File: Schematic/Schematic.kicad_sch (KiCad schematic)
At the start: 17 parts, among them J1 XT60-M, T1 Telemetry, U1 Matek PDB, U2 DRV8838

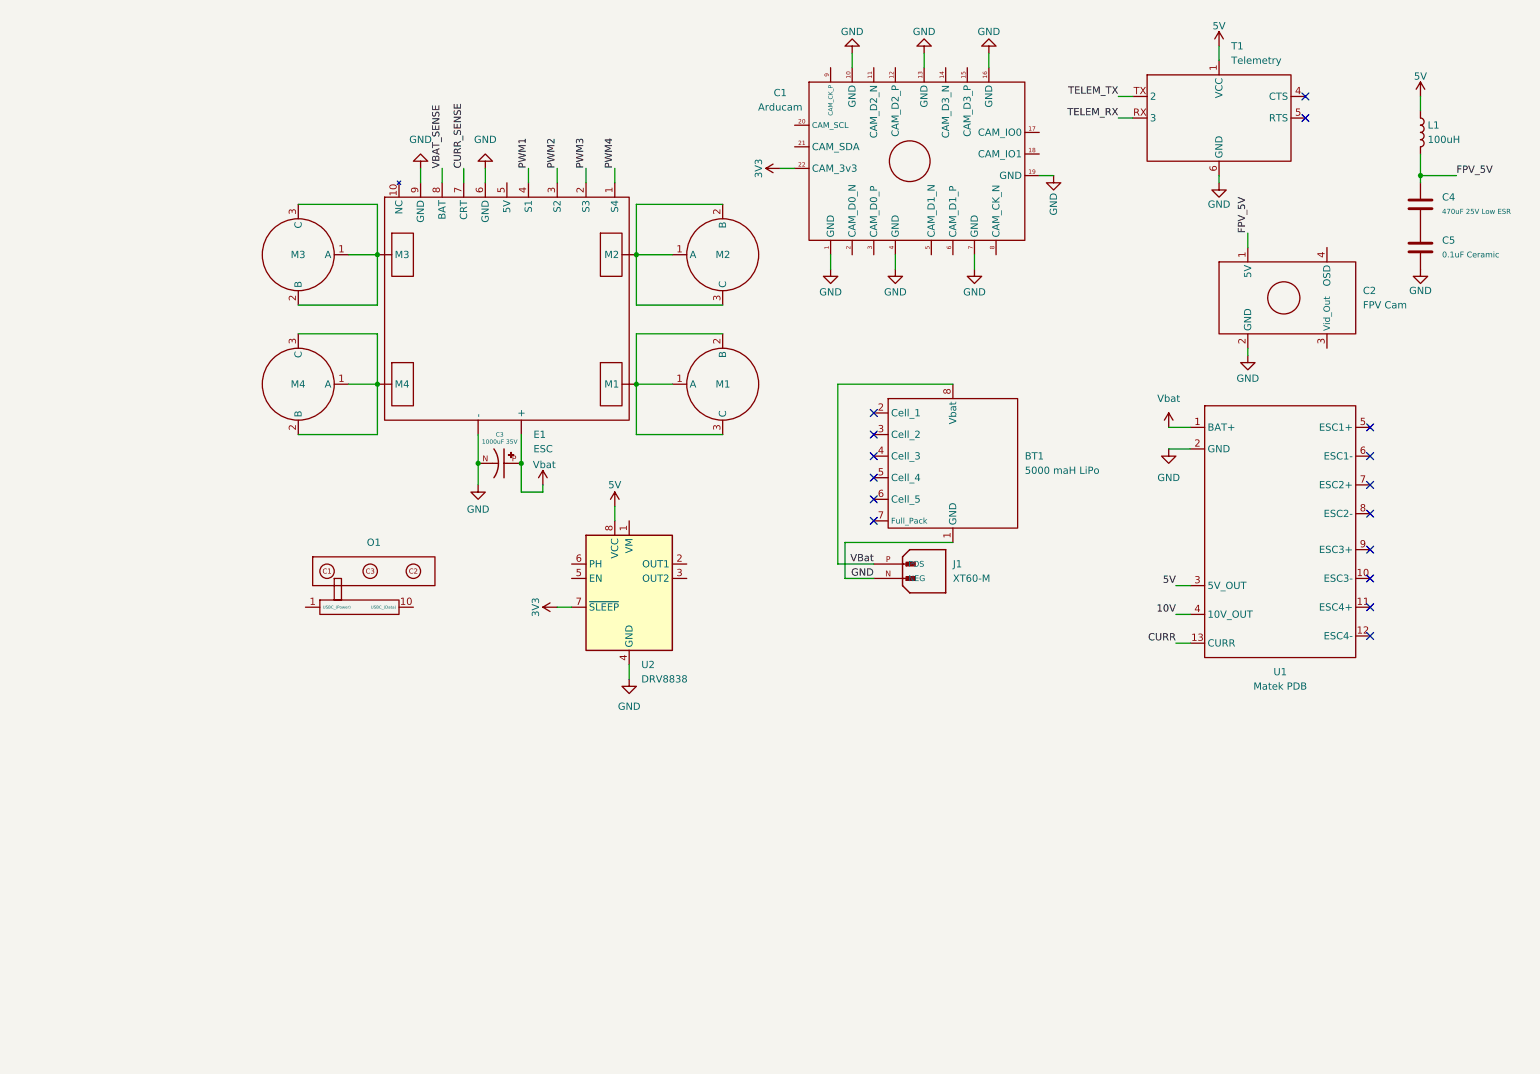
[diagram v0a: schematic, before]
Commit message: 6x and Jetson schematic
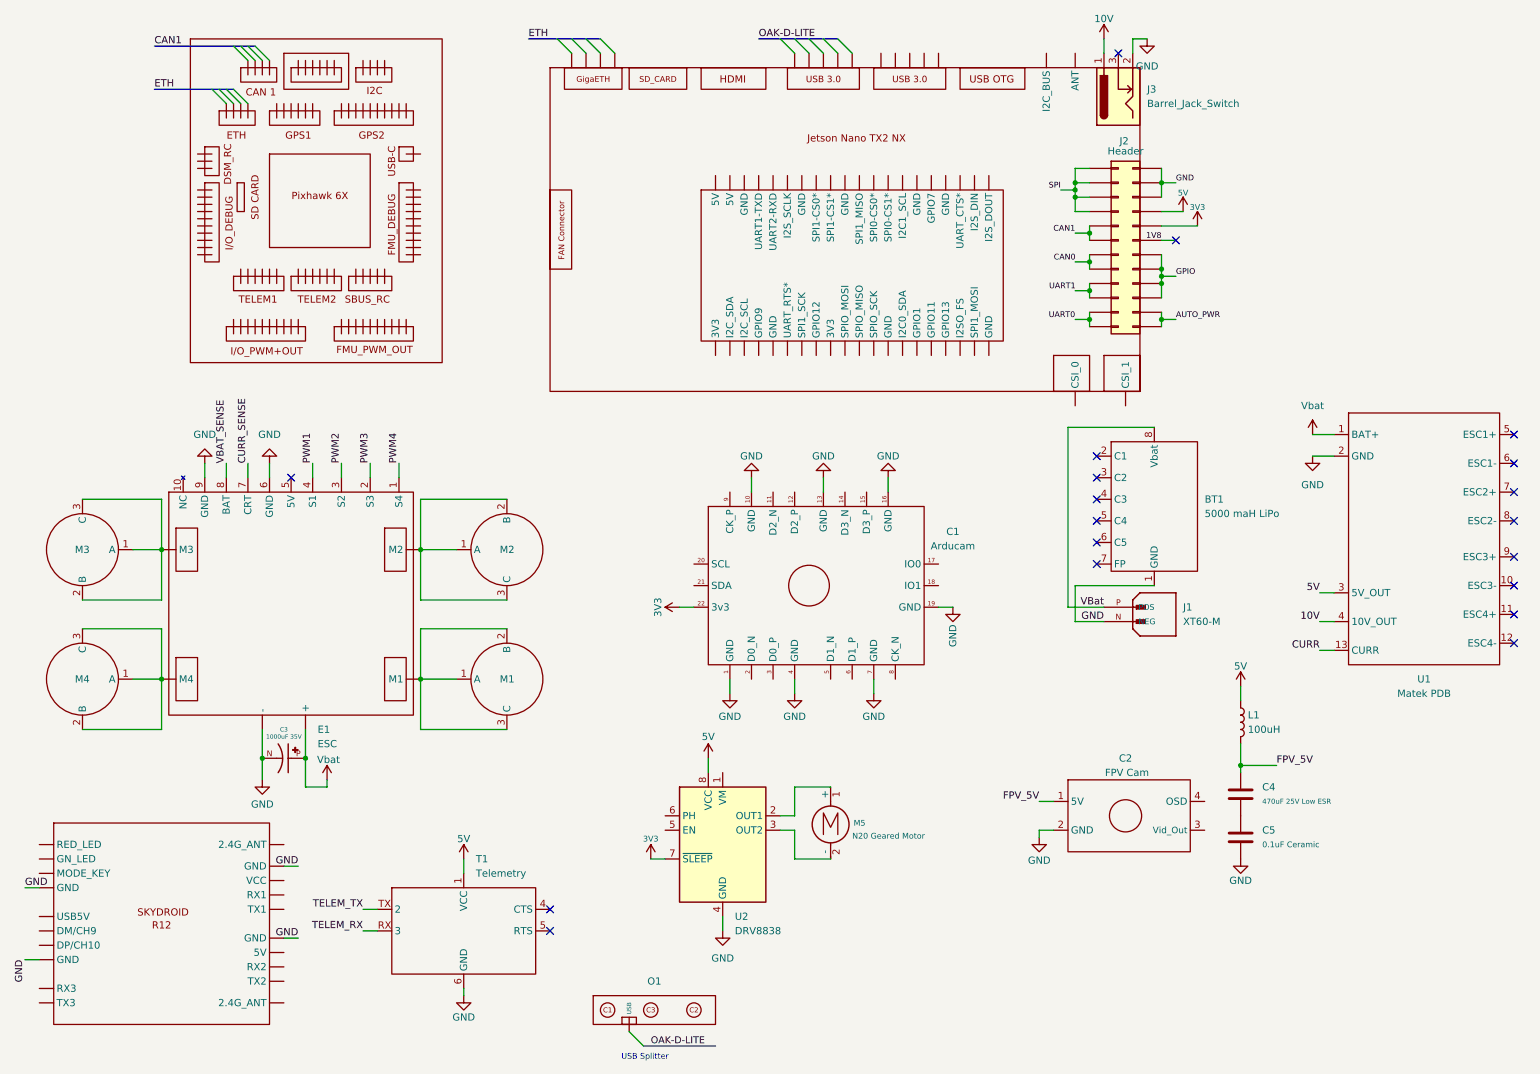
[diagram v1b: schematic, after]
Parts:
- added J2: Header, symbol Connector:DIN41612_02x10_AB
- added J3: Barrel_Jack_Switch, symbol Connector:Barrel_Jack_Switch
- added M5: N20 Geared Motor, symbol Motor:Motor_DC
- added U3: (no value), symbol Aerothon_custom-2:Pixahawk_6X_Mini_baseboard
- added U4: (no value), symbol Aerothon_custom-2:Skydroid R12
- added U5: (no value), symbol Aerothon_custom-2:Jetson_Nano
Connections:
- net 10V: now also J3.1
- net 3V3: now also J2. (Pin_b10)
- net 5V: now also J2. (Pin_b10)
- net GND: now also J2. (Pin_b10), J3.2, U4. (2.4G_ANT)
- net at U2.2 (OUT1): now also M5.1 (+)
- net at U2.3 (OUT2): now also M5.2 (-)
- new net 1V8: J2. (Pin_b10)
- new net AUTO_PWR: J2. (Pin_b10)
- new net CAN0: J2. (Pin_b10)
- new net CAN1: J2. (Pin_b10)
- new net GPIO: J2. (Pin_b10)
- new net SPI: J2. (Pin_b10)
- new net UART0: J2. (Pin_b10)
- new net UART1: J2. (Pin_b10)
- no-connect marks 16 -> 19
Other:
- note added: "USB Splitter"
- moved on the sheet: BT1, C1, C2, C3, C4, C5, E1, J1, L1, M1, M2, M3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
